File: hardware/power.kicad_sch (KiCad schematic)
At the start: 27 parts, among them J6 USB_C_Receptacle, Q1 DMG2307L, Q2 DMG2307L, Q3 BSD235N, U7 AP9101CK, U8 MIC5504-3.3YM5

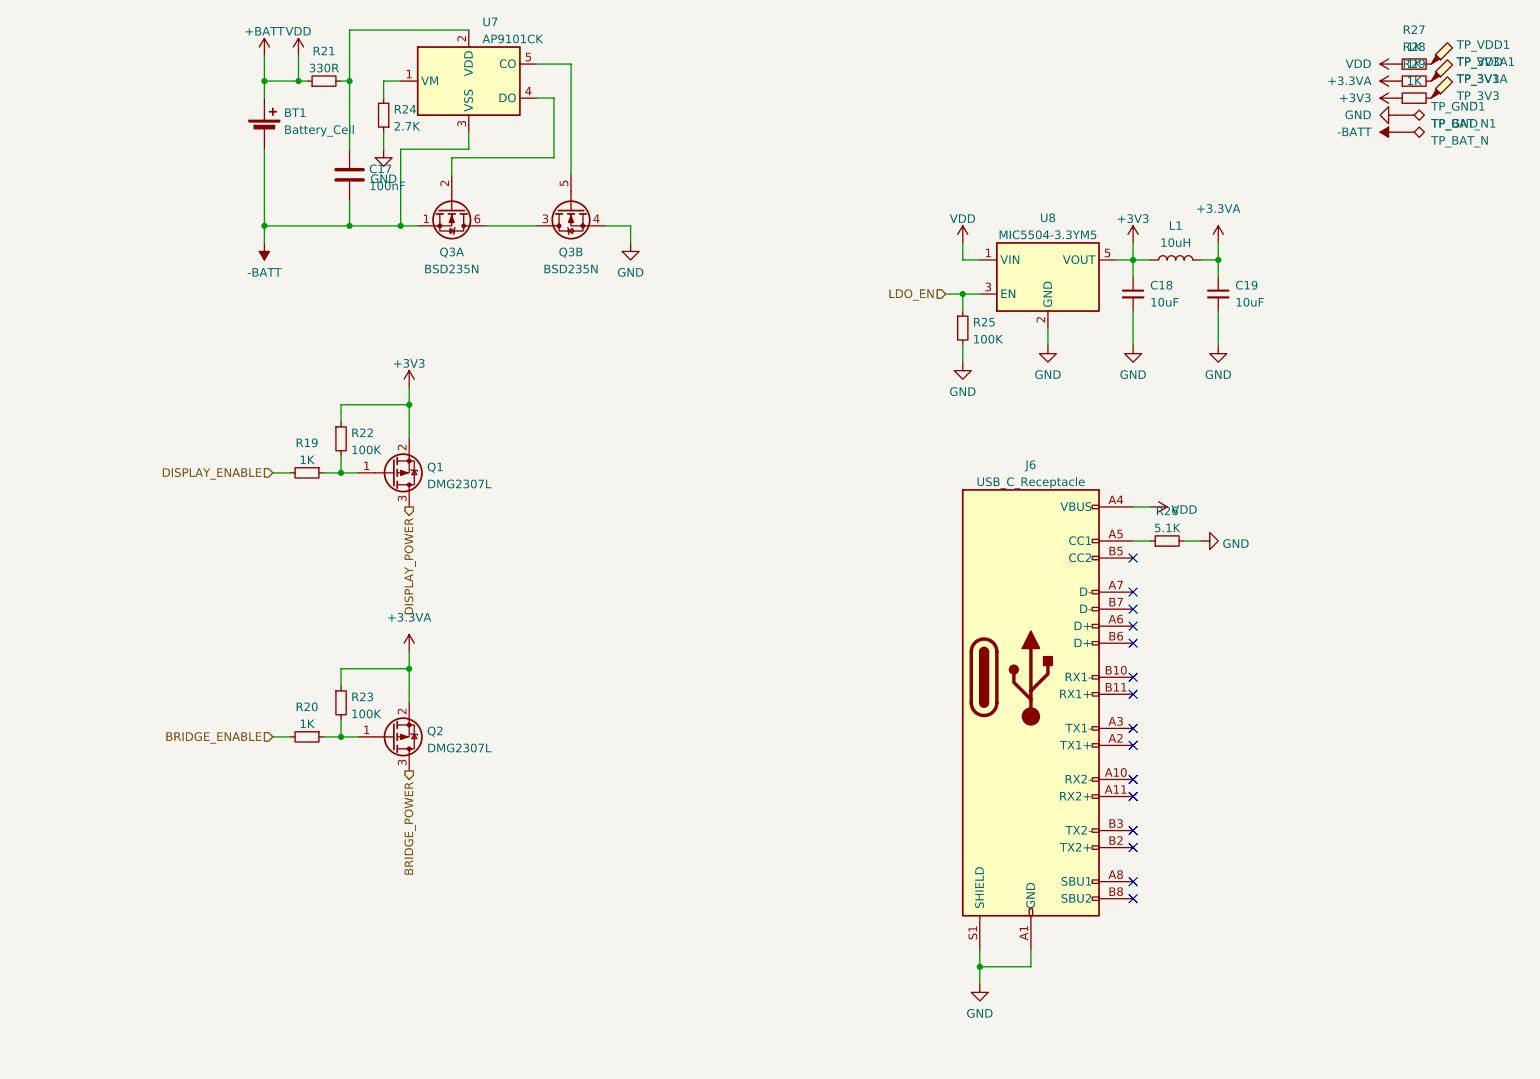
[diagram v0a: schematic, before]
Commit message: Major changes to schematic
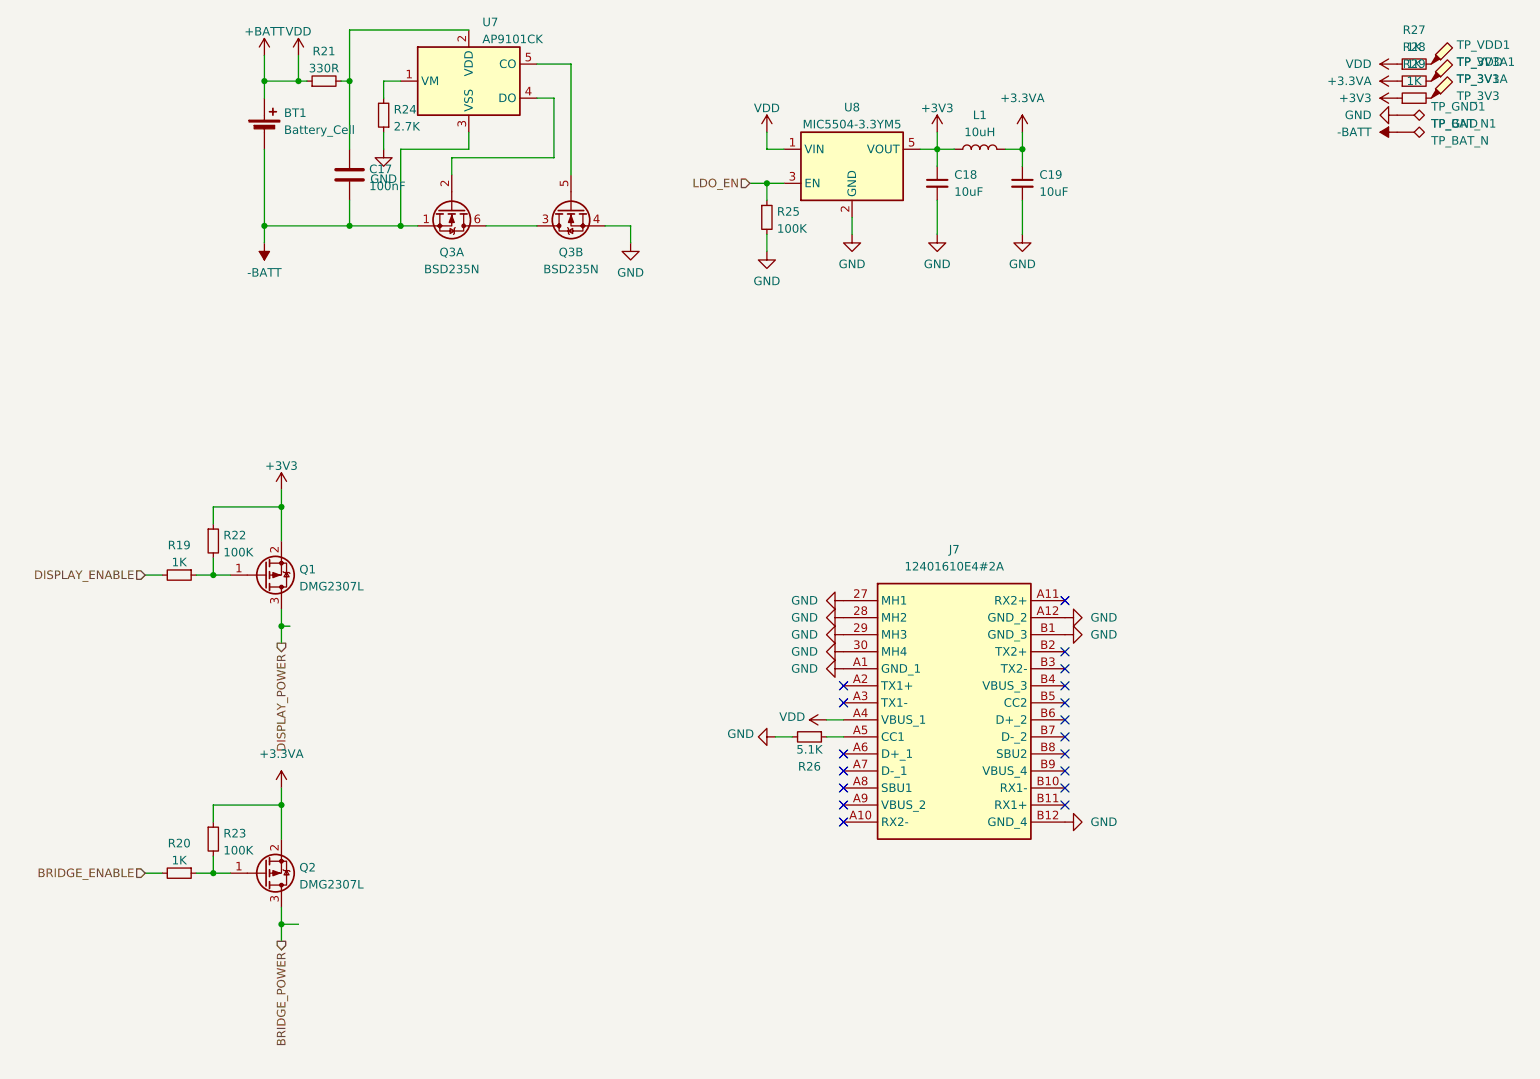
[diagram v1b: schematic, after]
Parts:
- removed J6: USB_C_Receptacle, Custom:USB_C_Receptacle_Amphenol_12401610E4-2A, symbol Connector:USB_C_Receptacle
- added J7: 12401610E4#2A, custom:12401610E42A, symbol 12401610E4#2A:12401610E4#2A
- C17: footprint Capacitor_SMD:C_0603_1608Metric_Pad1.08x0.95mm_HandSolder -> Capacitor_SMD:C_0603_1608Metric
- C18, C19: footprint (none) -> Capacitor_SMD:C_1210_3225Metric
- L1: footprint (none) -> Inductor_SMD:L_1210_3225Metric
- R19, R20, R21, R22, R23, R24, R25, R26, R27, R28, R29: footprint Resistor_SMD:R_0603_1608Metric_Pad0.98x0.95mm_HandSolder -> Resistor_SMD:R_0603_1608Metric
- TP_3V1, TP_3V3A1, TP_BAT_N1, TP_GND1, TP_VDD1: footprint (none) -> TestPoint:TestPoint_Pad_D1.5mm
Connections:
- net +BATT: now also J7.A4 (VBUS_1)
- net GND: now also J7.27 (MH1), J7.28 (MH2), J7.29 (MH3), J7.30 (MH4), J7.A1 (GND_1), J7.A12 (GND_2), J7.B1 (GND_3), J7.B12 (GND_4)
- net at R26.1: now also J7.A5 (CC1)
- no-connect marks 15 -> 18
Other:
- moved on the sheet: C18, C19, L1, Q1, Q2, R19, R20, R22, R23, R25, R26, U8
